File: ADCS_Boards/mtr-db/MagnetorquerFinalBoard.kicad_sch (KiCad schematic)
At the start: 47 parts, among them J1 PC104_Connector, U1 X/Y_Coils, U2 Z_Coil

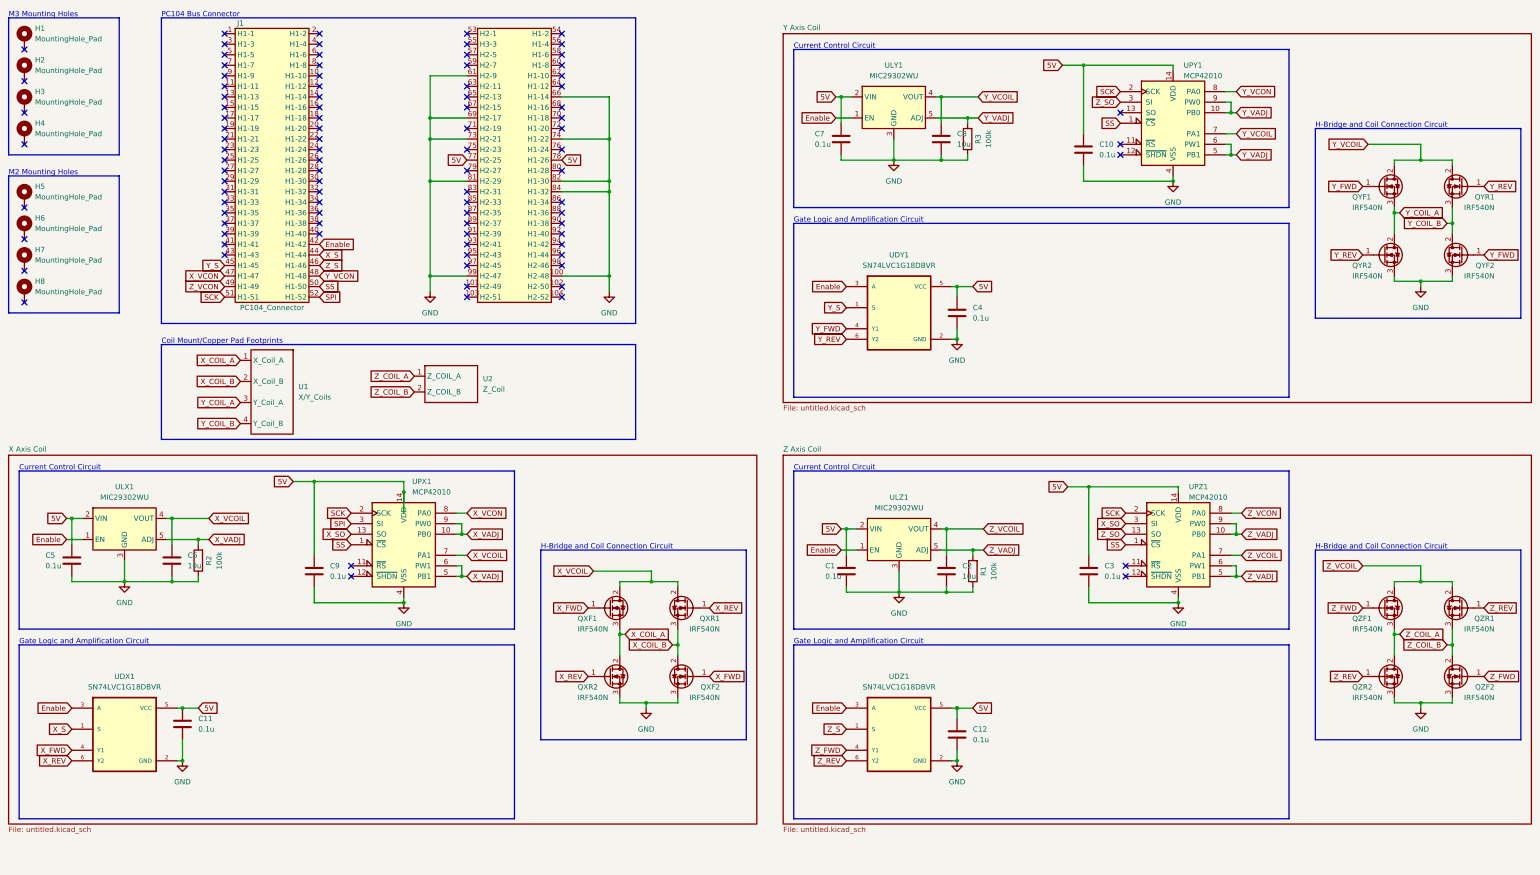
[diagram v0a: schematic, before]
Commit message: adcs: mtr-db: updated design from Liam
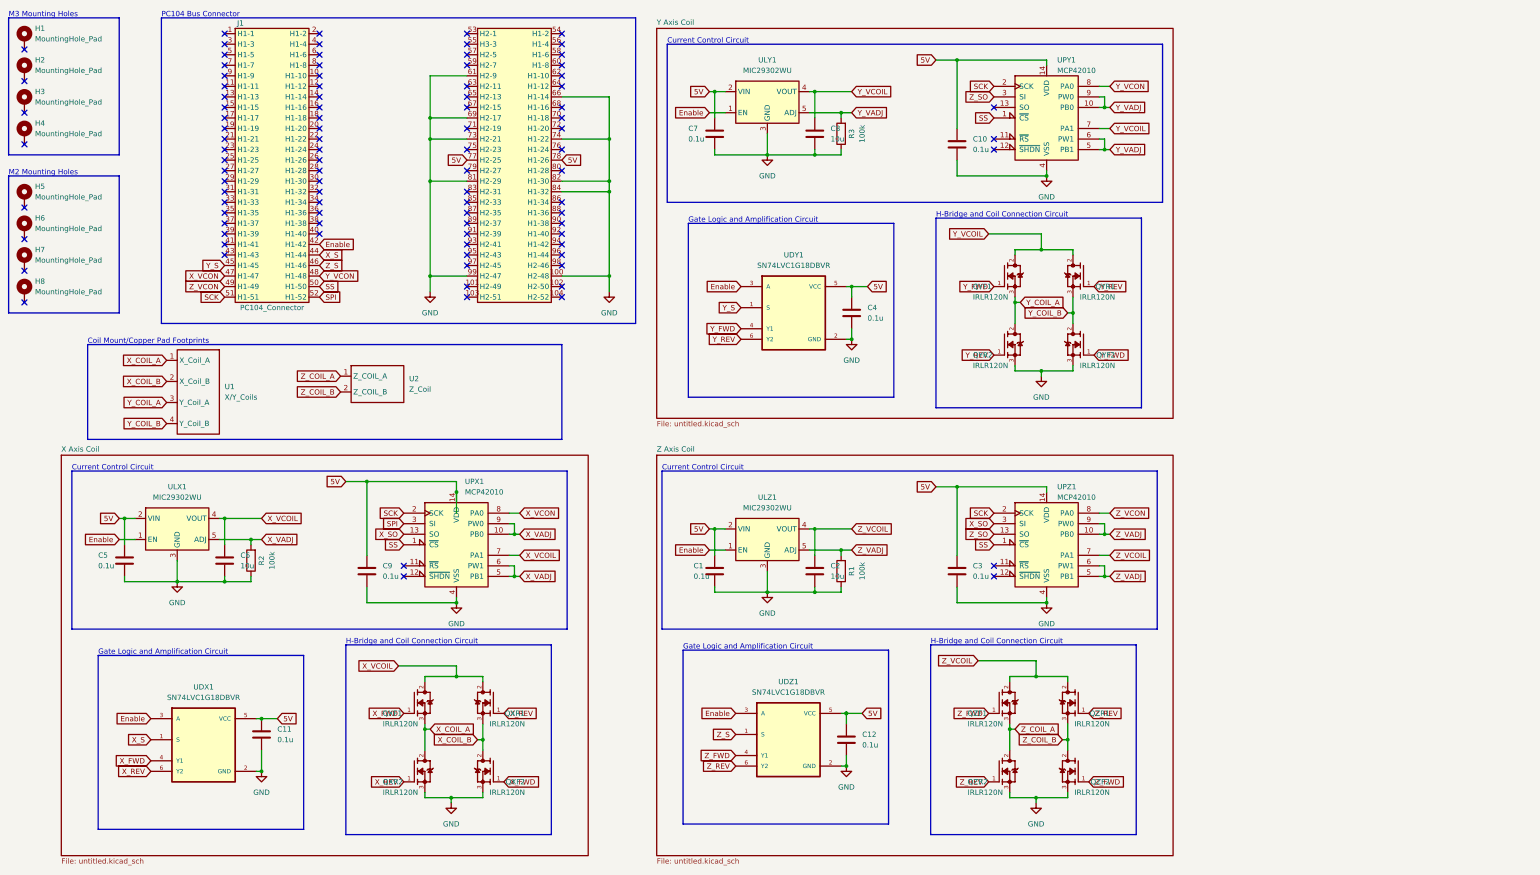
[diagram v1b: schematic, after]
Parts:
- QXF1, QXF2, QXR1, QXR2, QYF1, QYF2, QYR1, QYR2, QZF1, QZF2, QZR1, QZR2: value IRF540N -> IRLR120N; symbol Transistor_FET:IRF540N -> IRLR120N:IRLR120N; MANUFACTURER (none) -> Infineon Technologies; MAXIMUM_PACKAGE_HIEGHT (none) -> 2.39mm; PARTREV (none) -> july 2014; STANDARD (none) -> IPC7351B
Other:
- moved on the sheet: C1, C10, C11, C12, C2, C3, C4, C5, C6, C7, C8, C9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

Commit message: adcs: mtr-db: clean up schematic, include status LEDs in schematic
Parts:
- added D1, D2, D3, D4: ORANGE, LED_SMD:LED_0603_1608Metric, symbol Device:LED
- added JP1, JP2, JP3, JP4: SolderJumper_2_Open, Jumper:SolderJumper-2_P1.3mm_Open_TrianglePad1.0x1.5mm, symbol Jumper:SolderJumper_2_Open
- added R4, R5, R6, R7: 2k2, Resistor_SMD:R_0603_1608Metric, symbol Device:R
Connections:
- net 5V: now also D1.2 (A)
- net GND: now also JP1.1 (A), JP2.1 (A), JP3.1 (A), JP4.1 (A)
- net X_VCOIL: now also D2.2 (A)
- net Y_VCOIL: now also D4.2 (A)
- net Z_VCOIL: now also D3.2 (A)
- new net: JP2.2 (B), R6.2
- new net: D1.1 (K), R4.1
- new net: D3.1 (K), R6.1
- new net: JP1.2 (B), R4.2
- new net: D2.1 (K), R5.1
- new net: JP3.2 (B), R5.2
- new net: D4.1 (K), R7.1
- new net: JP4.2 (B), R7.2
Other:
- removed sheet X Axis Coil
- removed sheet Y Axis Coil
- removed sheet Z Axis Coil
- note added: "Status LEDs"
- note added: "X Axis Coil"
- note added: "Y Axis Coil"
- note added: "Z Axis Coil"
- moved on the sheet: C1, C10, C11, C12, C2, C3, C4, C5, C6, C7, C8, C9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
